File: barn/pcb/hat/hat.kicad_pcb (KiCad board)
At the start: 2 copper layers, 48 x 50.2 mm, 24 parts, among them J1 Conn_01x02, J2 Conn_01x02, J3 Conn_01x02, J4 Conn_01x02, J5 Conn_01x04, J6 Conn_02x13_Odd_Even, J7 Conn_01x13, J8 Conn_01x02, Q1 MMBT3904, Q2 MMBT3904, SW1 SW_Push_DPDT

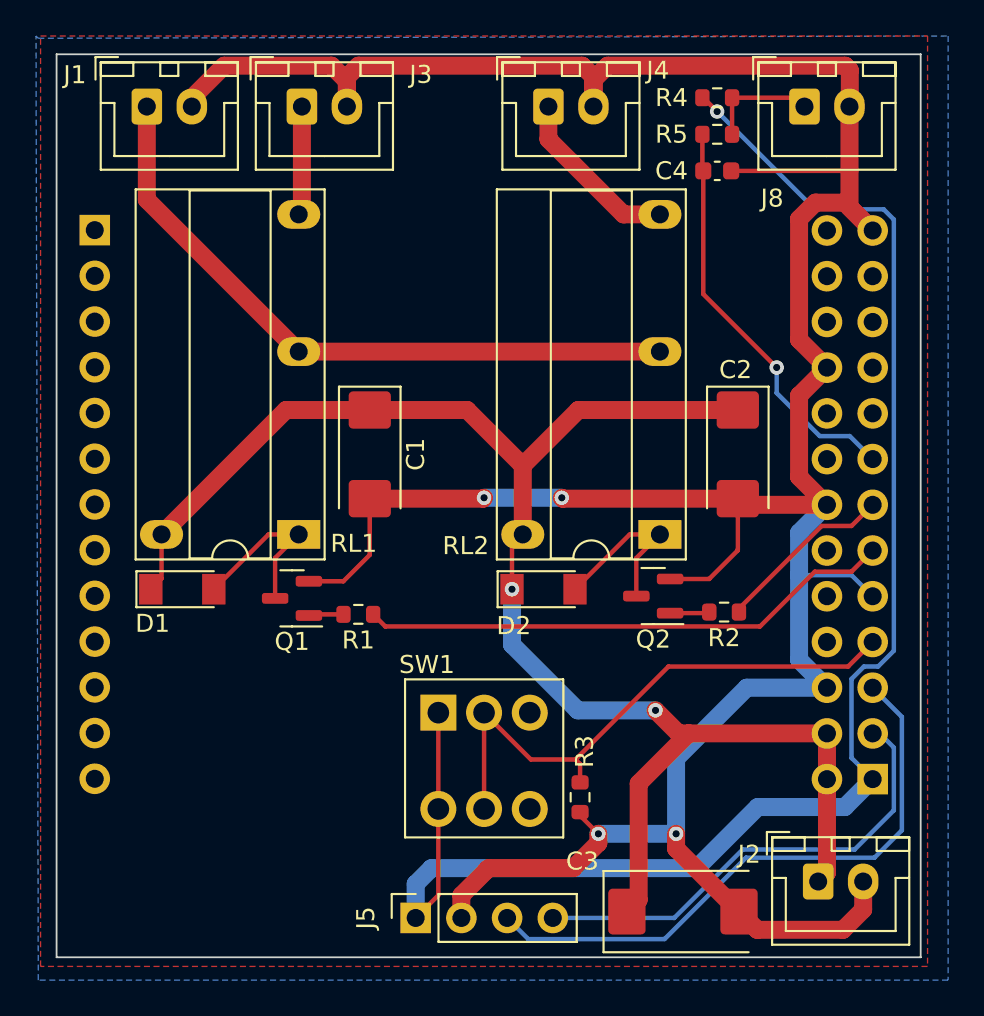
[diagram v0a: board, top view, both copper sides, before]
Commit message: Adjust edge cuts.
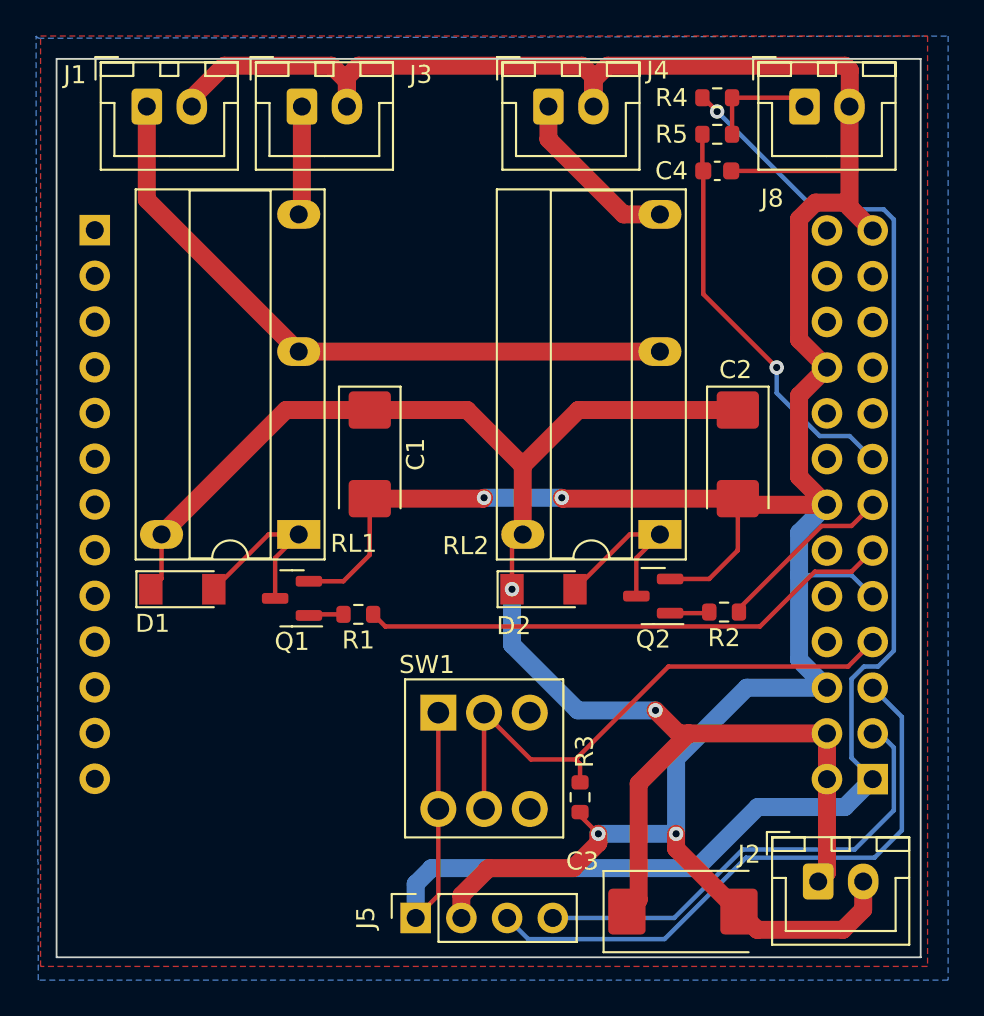
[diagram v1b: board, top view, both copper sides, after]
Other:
- board size 48 x 50.2 mm -> 48 x 49.9 mm
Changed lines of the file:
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@@
     )
   )
-  (gr_rect (start 47.879 70.231) (end 95.885 120.396) (layer "Edge.Cuts") (width 0.1) (fill none))
+  (gr_rect (start 47.879 70.485) (end 95.885 120.396) (layer "Edge.Cuts") (width 0.1) (fill none))
   (segment (start 90.678 107.96) (end 90.678 110.5) (width 1) (layer "F.Cu") (net 1))
   (segment (start 73.18 99.949) (end 73.18 97.503) (width 0.25) (layer "F.Cu") (net 1))
